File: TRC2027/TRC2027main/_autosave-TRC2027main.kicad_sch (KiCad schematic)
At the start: 55 parts, among them J1 Power_conn(XT90), J10 Memory, J11 BNO055, J12 Temperature, pressure, and al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, J13 Conn_01x03_Pin, J14 Conn_01x04_Pin, J15 Conn_01x04_Pin, J16 Conn_01x04_Pin, J17 Conn_01x04_Pin, J18 Conn_01x04_Pin, J19 Conn_01x12_Pin, J2 電圧計_測定, J20 Conn_01x10_Pin, J3 電圧計_電源, J4 XH_Moter_Output, J5 XH_Moter_Output, J6 Conn_01x07_Pin, J7 GPS, J8 Conn_01x08_Pin, J9 Conn_01x08_Pin, SW1 SW_SPST, U1 DCDC, U2 DRV8262DDWR, U3 DRV8262DDWR

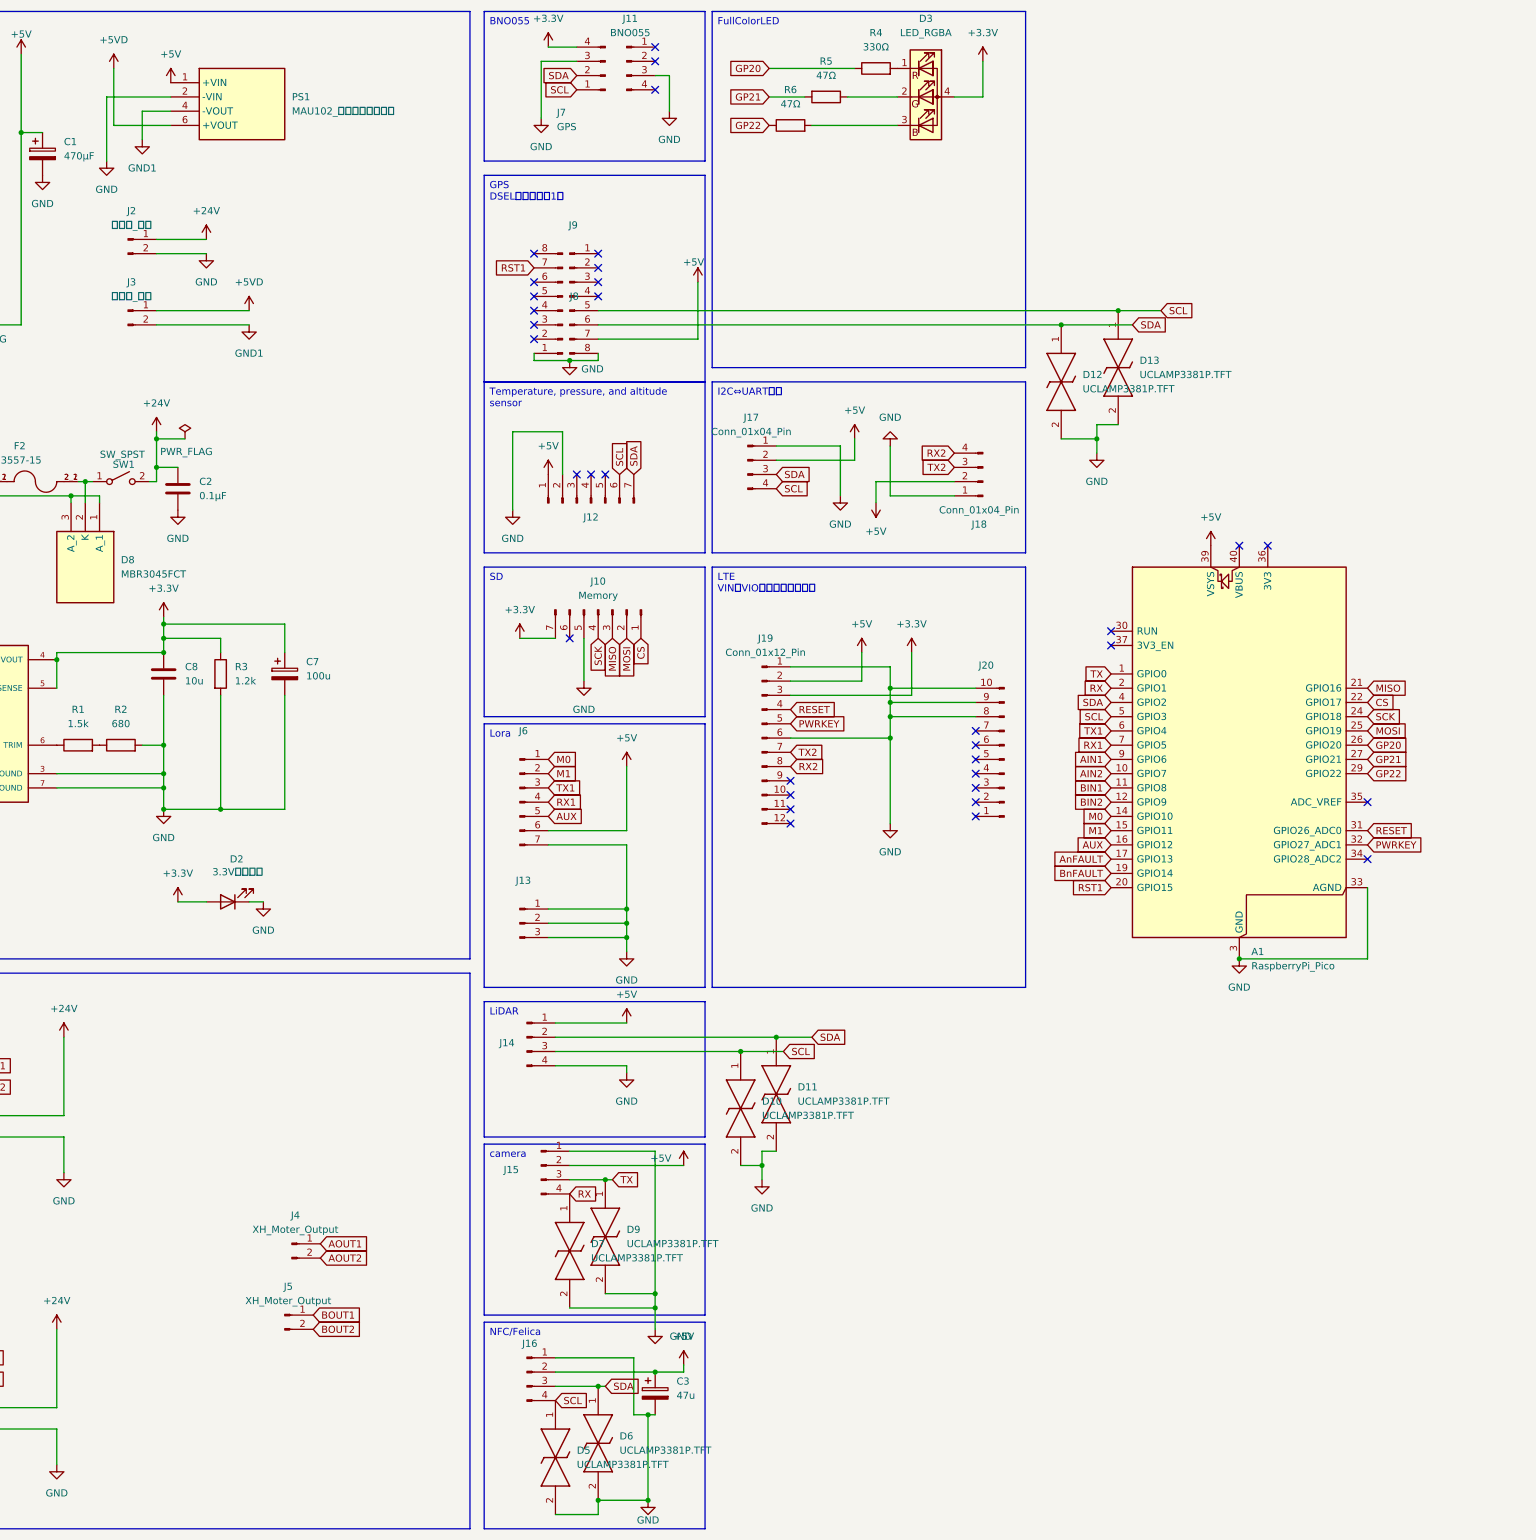
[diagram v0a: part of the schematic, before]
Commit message: change DataSheet
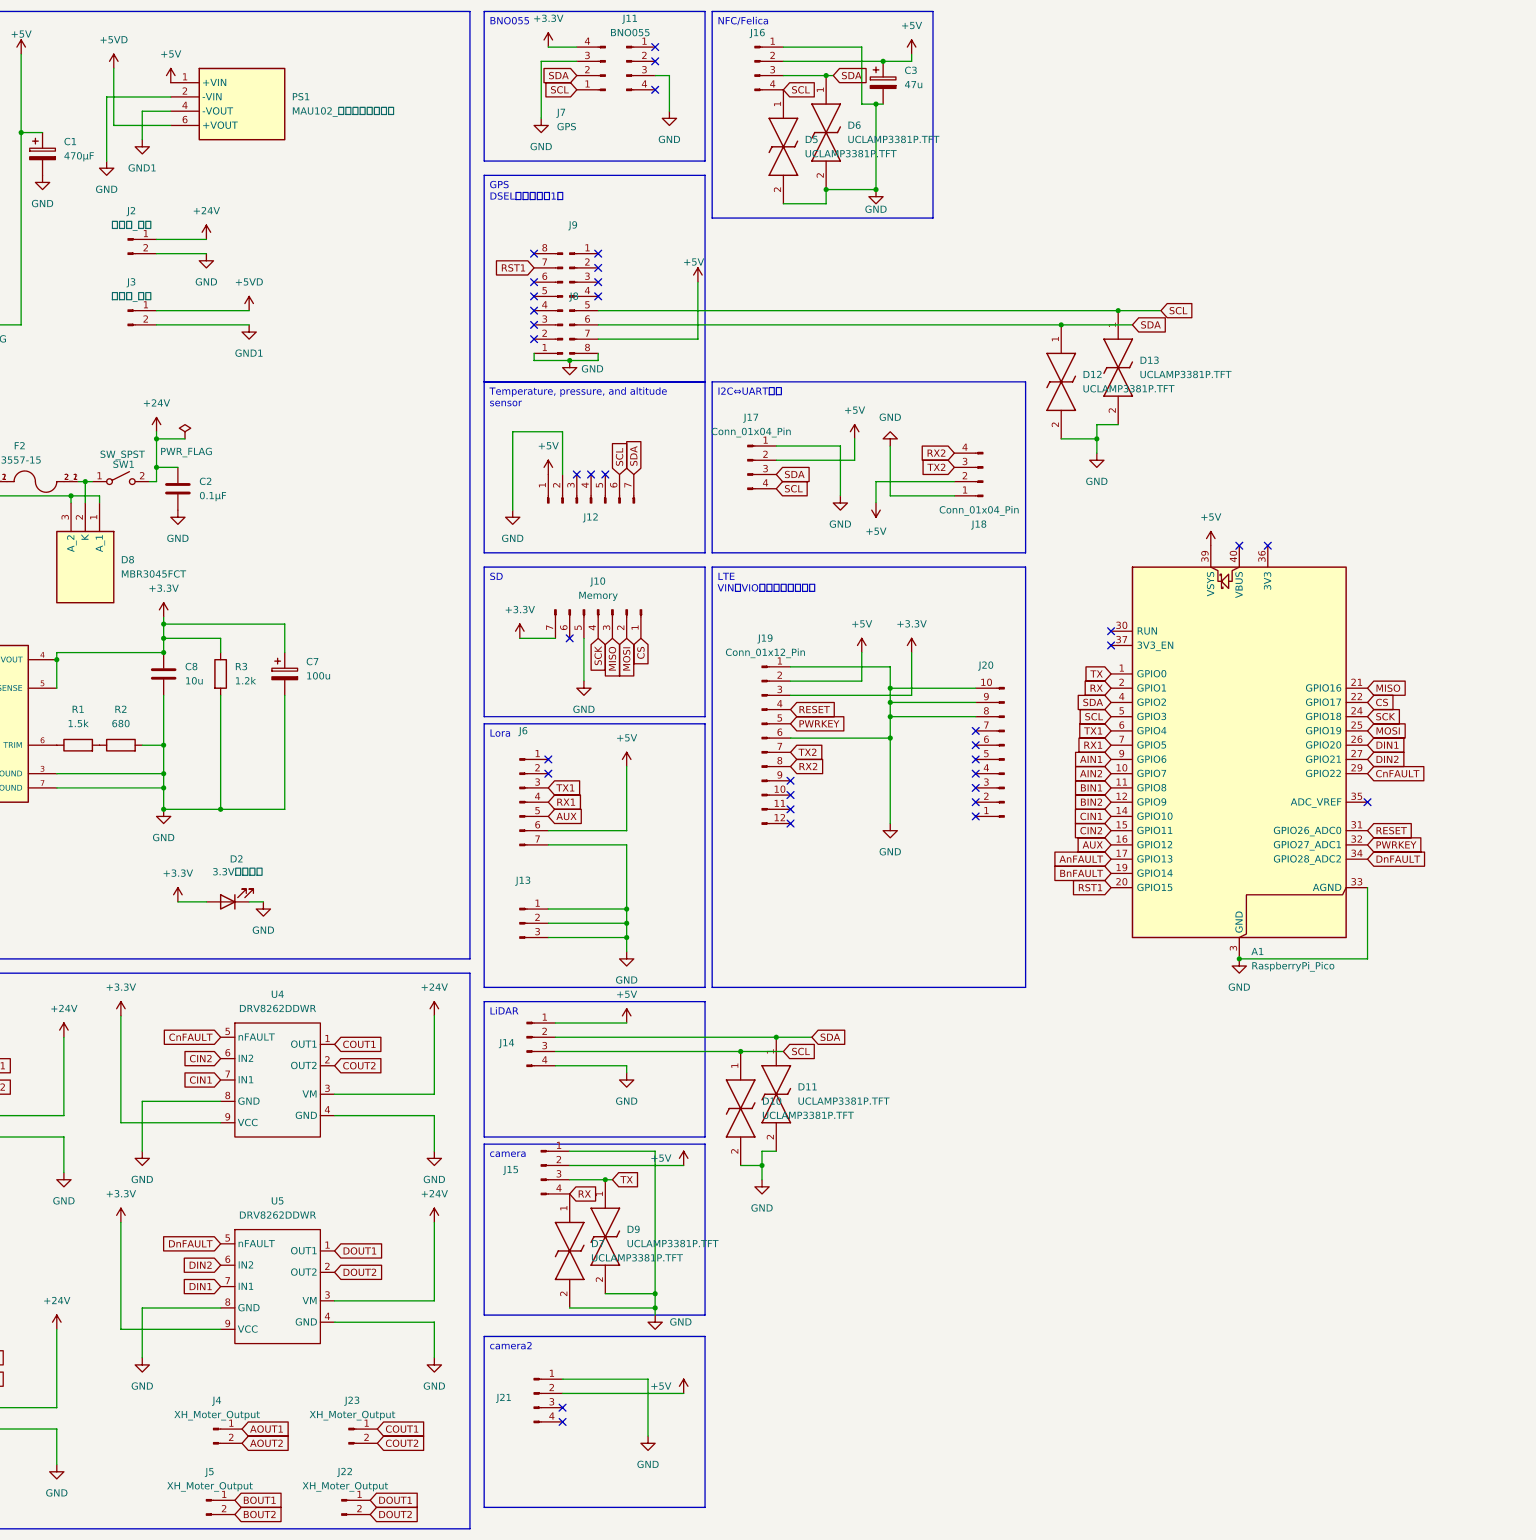
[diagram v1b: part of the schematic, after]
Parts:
- removed D3: LED_RGBA, symbol Device:LED_RGBA
- removed R4: 330Ω, symbol Device:R
- removed R5, R6: 47Ω, symbol Device:R
- added J21: Conn_01x04_Pin, symbol Connector:Conn_01x04_Pin
- added J22, J23: XH_Moter_Output, symbol Connector:Conn_01x02_Pin
- added U4, U5: DRV8262DDWR, symbol DRV8262DDWRModule:DRV8262DDWRModule
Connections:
- net +24V: now also U4.3 (VM), U5.3 (VM)
- net +3.3V: now also U4.9 (VCC), U5.9 (VCC)
- net +5V: now also J21.2 (Pin_2)
- net GND: now also J21.1 (Pin_1), U4.4 (GND), U4.8 (GND), U5.4 (GND), U5.8 (GND)
- net DnFAULT: now reaches A1.34 (GPIO28_ADC2)
- net DnFAULT: now also U5.5 (nFAULT)
- net GP20 renamed DIN1
- net DIN1: now also U5.7 (IN1)
- net GP21 renamed DIN2
- net DIN2: now also U5.6 (IN2)
- net GP22 renamed CnFAULT
- net CnFAULT: now also U4.5 (nFAULT)
- net M0: no longer names the net of J6.1 (Pin_1)
- net M0: no longer A1.14 (GPIO10)
- net M1: no longer names the net of J6.2 (Pin_2)
- net M1: no longer A1.15 (GPIO11)
- new net CIN1: A1.14 (GPIO10), U4.7 (IN1)
- new net CIN2: A1.15 (GPIO11), U4.6 (IN2)
- new net COUT1: J23.1 (Pin_1), U4.1 (OUT1)
- new net COUT2: J23.2 (Pin_2), U4.2 (OUT2)
- new net DOUT1: J22.1 (Pin_1), U5.1 (OUT1)
- new net DOUT2: J22.2 (Pin_2), U5.2 (OUT2)
- no-connect marks 44 -> 47
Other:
- moved on the sheet: C3, D5, D6, J16, J4, J5
